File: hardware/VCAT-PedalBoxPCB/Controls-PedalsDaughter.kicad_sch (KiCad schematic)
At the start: 21 parts, among them J1 MX150_02x03_Vertical, J6 MX150_02x10_Vertical

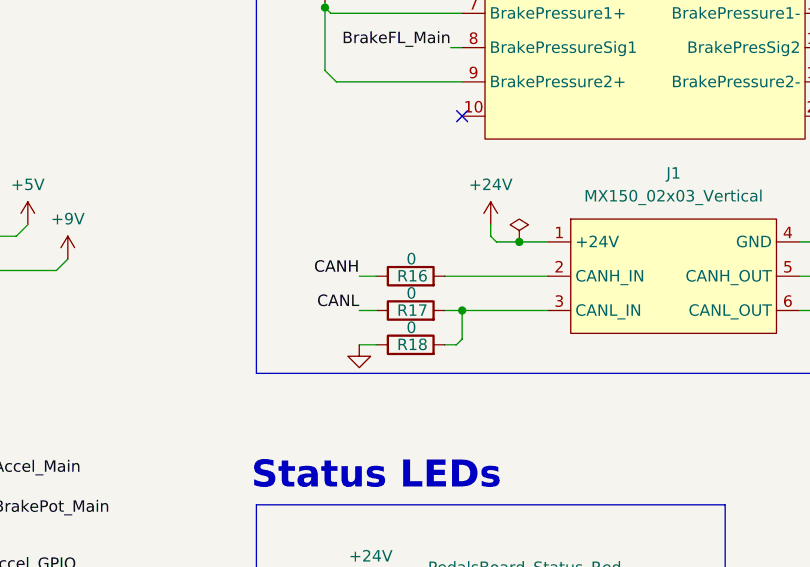
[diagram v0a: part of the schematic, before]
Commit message: Lakshay approved - final review #6
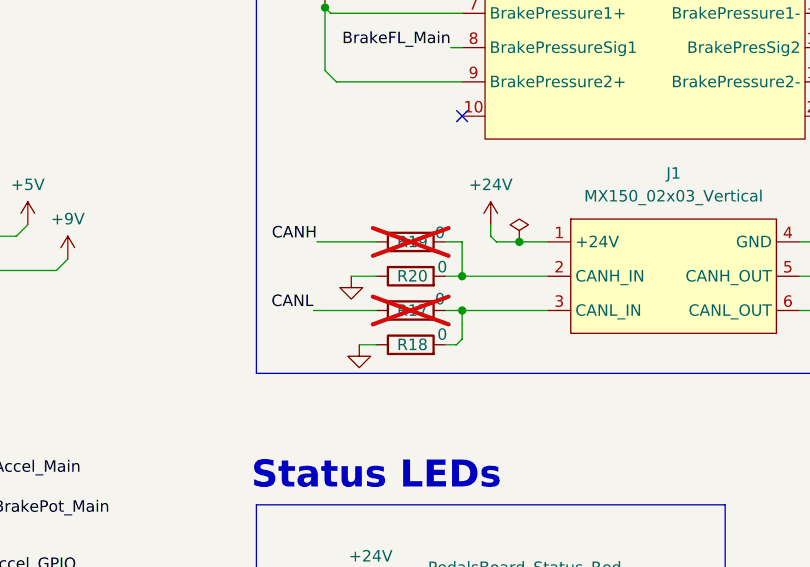
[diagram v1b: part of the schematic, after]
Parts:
- removed R16: 0, Resistor_SMD:R_0603_1608Metric_Pad0.98x0.95mm_HandSolder, symbol Device:R
- added R19, R20: 0, Resistor_SMD:R_0603_1608Metric_Pad0.98x0.95mm_HandSolder, symbol Device:R
- R17: now not fitted
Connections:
- net CANH: now also R19.1
- net GND: now also R20.1
- net at J1.2 (CANH_IN): now also R19.2, R20.2

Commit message: updated mx150 pin order :( works now
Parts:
- PSOM1: P/N 53307-2471 -> (none)
- R14, R15, R49: P/N FC0402E65R0BGT0 -> (none)
- R17, R18, R19, R20: P/N CRCW12101K10FKEAHP -> (none)

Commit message: updated BOM
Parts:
- J6: footprint UTSVT_Connectors:CONN_SD-75757-002_2X10_F16p09_MOL -> UTSVT_Connectors:MX150_02x10_Vertical
- R14, R15, R49: P/N (none) -> CRCW0603120RFKEC
- R17, R18, R19, R20: P/N (none) -> CRCW06030000Z0EE
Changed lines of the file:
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@@
 			)
 		)
-		(property "Description" "prgm LED"
+		(property "Description" "Pedals Status LEDs"
 			(at 122.555 153.035 0)
 			(effects
@@
 			)
 		)
-		(property "Description" ""
+		(property "Description" "Pedals CAN conn"
 			(at 142.24 93.345 0)
 			(effects
@@
 			)
 		)
-		(property "Description" "prgm led R45"
+		(property "Description" "Pedals status LED resistor"
 			(at 132.715 161.925 0)
 			(effects
@@
 			)
 		)
-		(property "P/N" ""
+		(property "P/N" "CRCW0603120RFKEC "
 			(at 132.715 161.925 90)
 			(effects
@@
 			)
 		)
-		(property "Description" "Controls R47"
+		(property "Description" "Pedals goofy ah 0 ohms"
 			(at 113.03 103.505 0)
 			(effects
@@
 			)
 		)
-		(property "P/N" "~"
+		(property "P/N" "CRCW06030000Z0EE"
 			(at 113.03 103.505 90)
 			(effects
@@
 			)
 		)
-		(property "Description" "Board-to-board connector for Peripheral SOM daughterboards"
+		(property "Description" "PSOM"
 			(at 229.235 35.814 0)
 			(effects
@@
 			)
 		)
+		(property "P/N" "~"
+			(at 184.15 152.4 90)
+			(effects
+				(font
+					(size 1.27 1.27)
+				)
+				(hide yes)
+			)
+		)
 		(pin "1"
 		)
@@
 			)
 		)
-		(property "Description" "Controls Lead LED"
+		(property "Description" "Pedals PWR LED"
 			(at 121.92 141.605 0)
 			(effects
@@
 			)
 		)
-		(property "Description" "Controls R47"
+		(property "Description" "Pedals PWR LED R47"
 			(at 132.08 141.605 0)
 			(effects
@@
 			)
 		)
-		(property "Footprint" "UTSVT_Connectors:CONN_SD-75757-002_2X10_F16p09_MOL"
+		(property "Footprint" "UTSVT_Connectors:MX150_02x10_Vertical"
 			(at 132.715 45.085 0)
 			(effects
@@
 			)
 		)
-		(property "Description" ""
+		(property "Description" "Pedals MX150"
 			(at 132.715 45.085 0)
 			(effects
@@
 			)
 		)
-		(property "Description" "prgm LED"
+		(property "Description" "Pedals Status LEDs"
 			(at 122.555 161.925 0)
 			(effects
@@
 			)
 		)
-		(property "Description" "prgm led R45"
+		(property "Description" "Pedals status LED resistor"
 			(at 132.715 153.035 0)
 			(effects
@@
 			)
 		)
-		(property "P/N" ""
+		(property "P/N" "CRCW0603120RFKEC "
 			(at 132.715 153.035 90)
 			(effects
@@
 			)
 		)
-		(property "Description" "Controls R47"
+		(property "Description" "Pedals goofy ah 0 ohms"
 			(at 113.03 107.315 0)
 			(effects
@@
 			)
 		)
-		(property "P/N" "~"
+		(property "P/N" "CRCW06030000Z0EE"
 			(at 113.03 107.315 90)
 			(effects
@@
 			)
 		)
-		(property "Description" "prgm led R45"
+		(property "Description" "Pedals status LED resistor"
 			(at 133.35 170.18 0)
 			(effects
@@
 			)
 		)
-		(property "P/N" ""
+		(property "P/N" "CRCW0603120RFKEC "
 			(at 133.35 170.18 90)
 			(effects
@@
 			)
 		)
-		(property "Description" "prgm LED"
+		(property "Description" "Pedals Status LEDs"
 			(at 123.19 170.18 0)
 			(effects
@@
 			)
 		)
-		(property "Description" "Controls R47"
+		(property "Description" "Pedals goofy ah 0 ohms"
 			(at 113.03 111.125 0)
 			(effects
@@
 			)
 		)
-		(property "P/N" "~"
+		(property "P/N" "CRCW06030000Z0EE"
 			(at 113.03 111.125 90)
 			(effects
@@
 			)
 		)
-		(property "Description" "Controls R47"
+		(property "Description" "Pedals goofy ah 0 ohms"
 			(at 113.03 99.695 0)
 			(effects
@@
 			)
 		)
-		(property "P/N" "~"
+		(property "P/N" "CRCW06030000Z0EE"
 			(at 113.03 99.695 90)
 			(effects

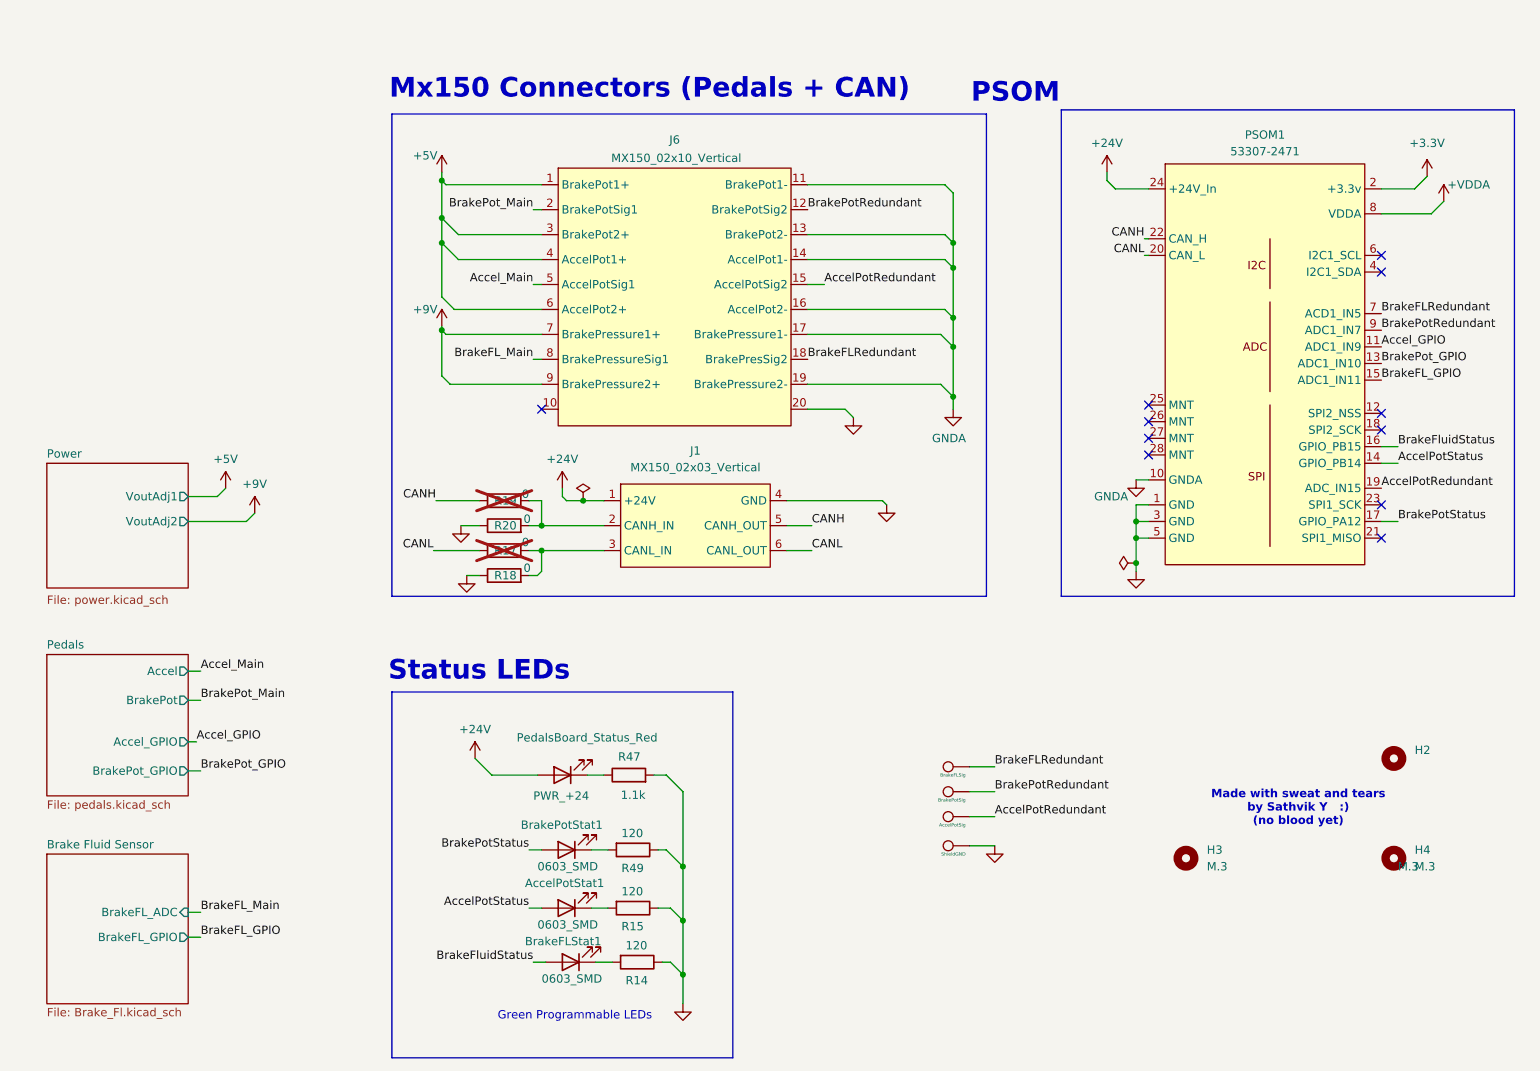
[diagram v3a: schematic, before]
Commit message: Final review..(?)
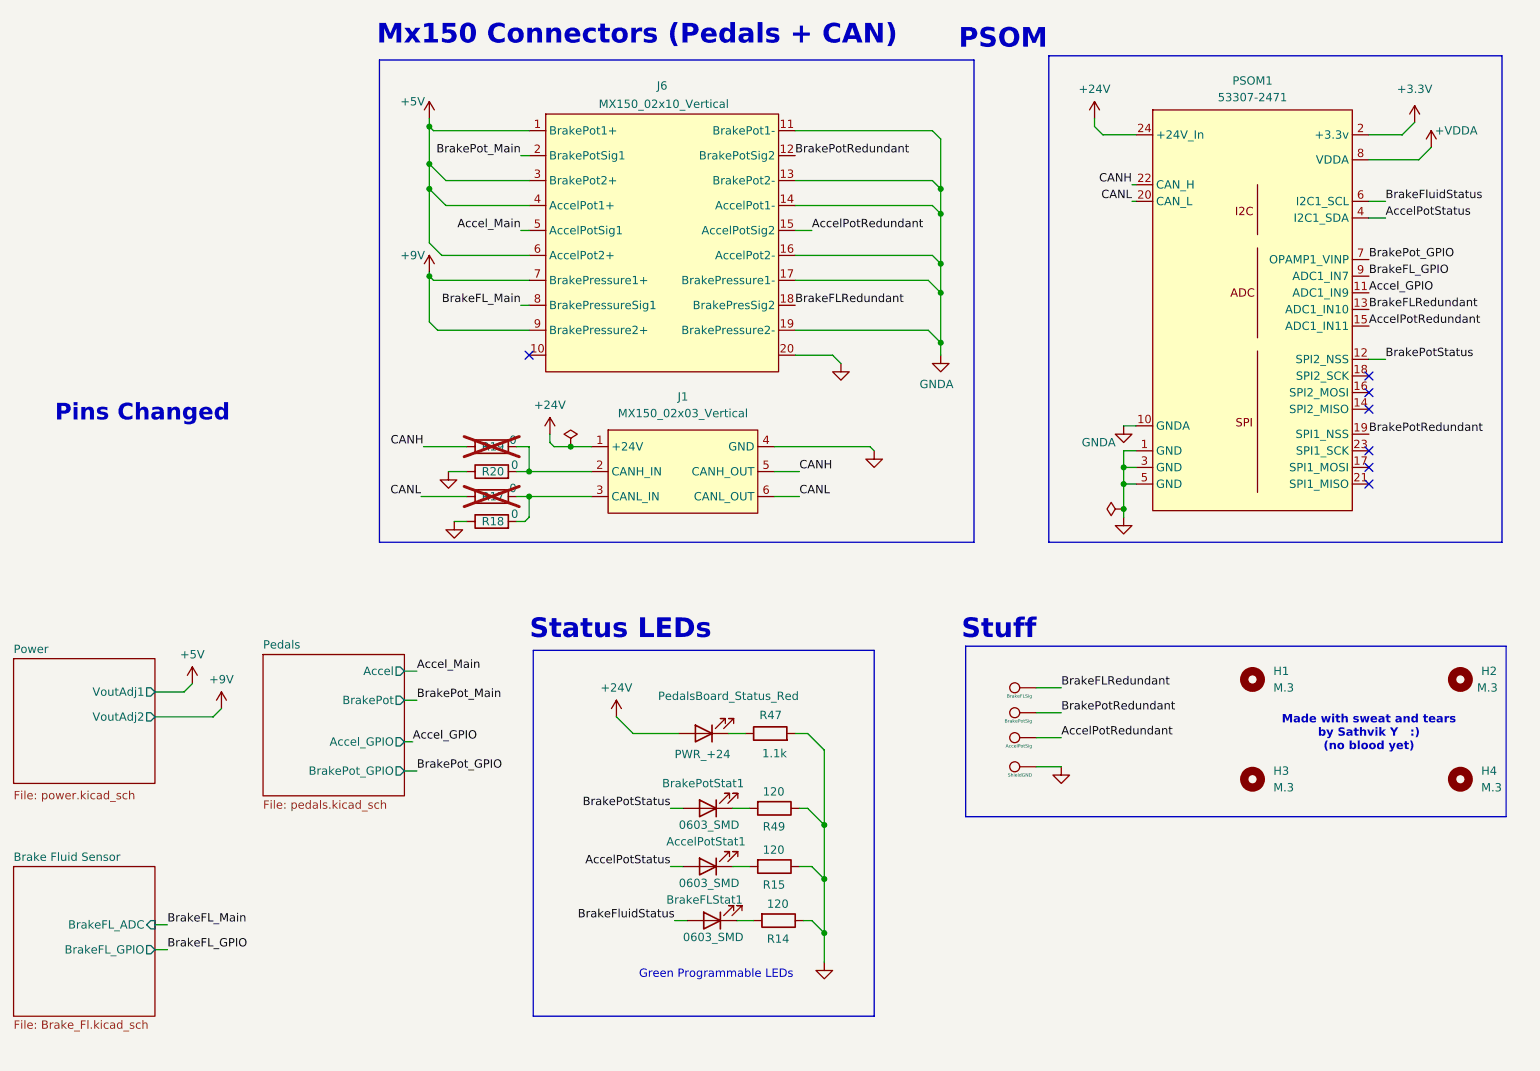
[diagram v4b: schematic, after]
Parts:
- added H1: M.3, MountingHole:MountingHole_3.2mm_M3_Pad_TopBottom, symbol Mechanical:MountingHole
- PSOM1: P/N (none) -> 53307-2471
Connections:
- net AccelPotRedundant: now also PSOM1.15 (ADC1_IN11); no longer PSOM1.19 (ADC_IN15)
- net AccelPotStatus: now also PSOM1.4 (I2C1_SDA); no longer PSOM1.14 (GPIO_PB14)
- net BrakeFLRedundant: now also PSOM1.13 (ADC1_IN10); no longer PSOM1.7 (ACD1_IN5)
- net BrakeFL_GPIO: now also PSOM1.9 (ADC1_IN7); no longer PSOM1.15 (ADC1_IN11)
- net BrakeFluidStatus: now also PSOM1.6 (I2C1_SCL); no longer PSOM1.16 (GPIO_PB15)
- net BrakePotRedundant: now also PSOM1.19 (SPI1_NSS); no longer PSOM1.9 (ADC1_IN7)
- net BrakePotStatus: now also PSOM1.12 (SPI2_NSS); no longer PSOM1.17 (GPIO_PA12)
- net BrakePot_GPIO: now also PSOM1.7 (OPAMP1_VINP); no longer PSOM1.13 (ADC1_IN10)
- no-connect marks 11 -> 7
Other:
- note added: "Pins Changed"
- note added: "Stuff"
- moved on the sheet: AccelPotStat1, BrakeFLStat1, BrakePotStat1, H2, H3, H4, J1, J6, PWR_+24, R14, R15, R17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
